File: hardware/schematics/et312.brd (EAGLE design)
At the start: 160 x 100 mm, 119 parts, among them IC1 LM324N, IC2 4066N, IC3 LM358, IC4 7809, IC5 LM358N, IC6 7809, J1 BATTERY_CONNDEANS, Q1 IRL520N-H, Q2 IRL520N-H, Q3 IRF9Z24, Q4 IRL520N-H, Q5 IRL520N-H, Q6 IRF9Z24, Q7 2N3906, T1 2N3904, U1 MEGA16-P, U9 7805, X1 HD44780LCD-1602, X2 STEREOJACK, X3 STEREOJACK, X4 STEREOJACK, X5 STEREOJACK, X6 STEREOJACK

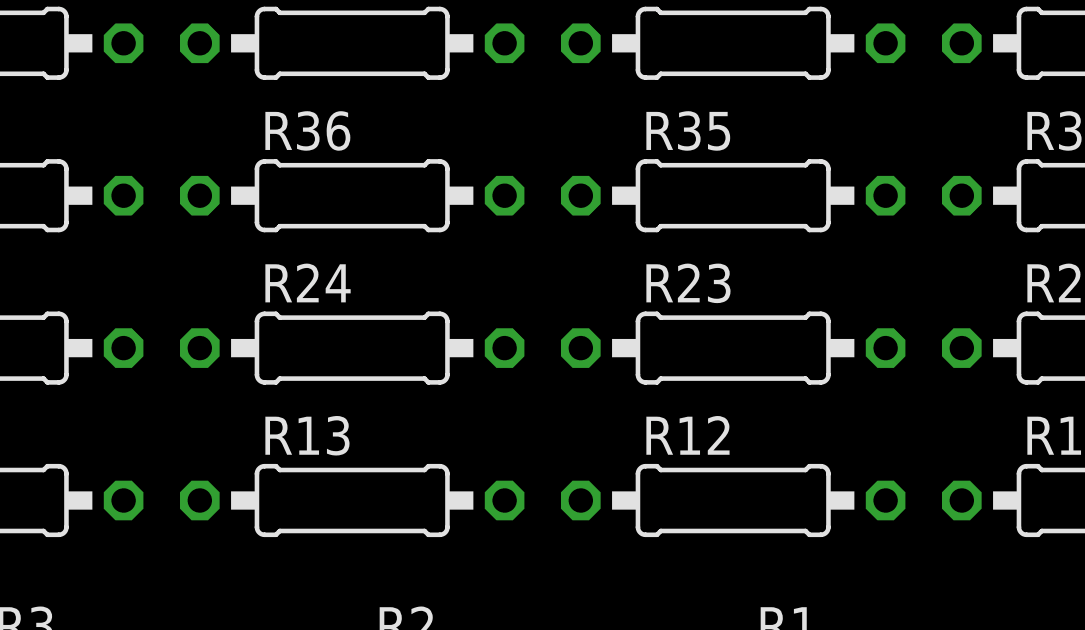
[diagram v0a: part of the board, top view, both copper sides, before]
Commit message: Arduino Sheild Eagle
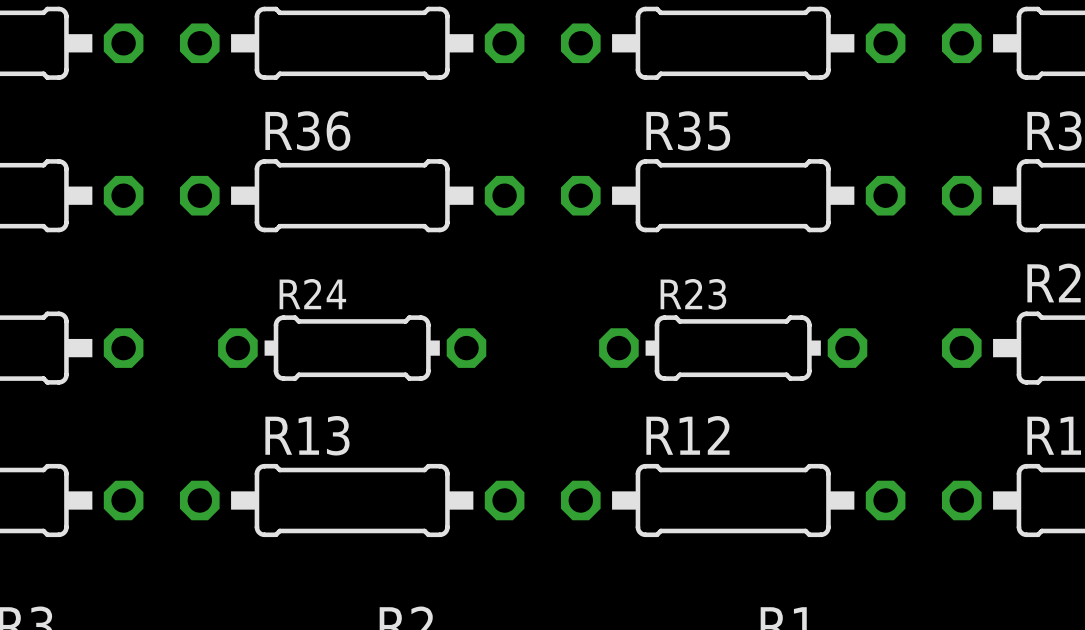
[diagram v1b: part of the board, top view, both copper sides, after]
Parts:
- R23, R24: device rcl:0207/10 -> rcl:0204/7
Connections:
- net +12V: no longer C7.+, L1.2
- net N$31: now also C7.+, L1.2; no longer L1.1
- net V+: now also L1.1
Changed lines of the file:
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@@
 <?xml version="1.0" encoding="utf-8"?>
 <!DOCTYPE eagle SYSTEM "eagle.dtd">
-<eagle version="7.3.0">
+<eagle version="7.1.0">
 <drawing>
 <settings>
@@
 <attribute name="SPICEPREFIX" value="R" x="-44.45" y="147.32" size="1.778" layer="27" display="off"/>
 </element>
-<element name="R23" library="rcl" package="0207/10" value="" x="-57.15" y="147.32"/>
-<element name="R24" library="rcl" package="0207/10" value="" x="-69.85" y="147.32"/>
+<element name="R23" library="rcl" package="0204/7" value="" x="-57.15" y="147.32"/>
+<element name="R24" library="rcl" package="0204/7" value="" x="-69.85" y="147.32"/>
 <element name="R25" library="pot" package="LI10" value="" x="-19.05" y="110.49"/>
 <element name="R26" library="rcl" package="0207/10" value="390R" x="-82.55" y="147.32"/>
@@
 <contactref element="IC1" pad="4"/>
 <contactref element="IC5" pad="8"/>
+<contactref element="RP6" pad="2"/>
 <contactref element="JP1" pad="PWR"/>
+<contactref element="U$1" pad="4"/>
 <contactref element="C5" pad="+"/>
-<contactref element="U$1" pad="4"/>
-<contactref element="RP6" pad="2"/>
-<wire x1="-71.12" y1="105.41" x2="-22.86" y2="125.73" width="0" layer="19" extent="1-1"/>
+<contactref element="L1" pad="1"/>
+<wire x1="-45.72" y1="135.89" x2="-22.86" y2="125.73" width="0" layer="19" extent="1-1"/>
+<wire x1="-64.77" y1="162.56" x2="-45.72" y2="135.89" width="0" layer="19" extent="1-1"/>
+<wire x1="-71.12" y1="105.41" x2="-45.72" y2="135.89" width="0" layer="19" extent="1-1"/>
 <wire x1="-101.6" y1="130.81" x2="-71.12" y2="105.41" width="0" layer="19" extent="1-1"/>
-<wire x1="-64.77" y1="162.56" x2="-101.6" y2="130.81" width="0" layer="19" extent="1-1"/>
 <wire x1="-99.02" y1="53.17" x2="-71.12" y2="105.41" width="0" layer="19" extent="1-1"/>
 <wire x1="-110.0582" y1="40.64" x2="-99.02" y2="53.17" width="0" layer="19" extent="1-1"/>
@@
 <contactref element="C4" pad="2"/>
 <contactref element="IC6" pad="2"/>
-<contactref element="JP1" pad="GND@1"/>
-<contactref element="JP1" pad="GND@2"/>
-<contactref element="C5" pad="-"/>
-<contactref element="U$1" pad="3"/>
-<contactref element="U$1" pad="2"/>
 <contactref element="R24" pad="1"/>
 <contactref element="C6" pad="-"/>
 <contactref element="C8" pad="2"/>
-<contactref element="J1" pad="-"/>
 <contactref element="C7" pad="-"/>
 <contactref element="U1" pad="11"/>
@@
 <contactref element="U$2" pad="1"/>
 <contactref element="R52" pad="1"/>
+<contactref element="JP1" pad="GND@2"/>
+<contactref element="JP1" pad="GND@1"/>
+<contactref element="U$1" pad="2"/>
+<contactref element="U$1" pad="3"/>
+<contactref element="C5" pad="-"/>
+<contactref element="J1" pad="-"/>
 <wire x1="-13.97" y1="152.4" x2="-13.97" y2="157.48" width="0" layer="19" extent="1-1"/>
 <wire x1="-24.13" y1="147.32" x2="-13.97" y2="152.4" width="0" layer="19" extent="1-1"/>
@@
 <wire x1="-62.23" y1="142.24" x2="-58.42" y2="135.89" width="0" layer="19" extent="1-1"/>
 <wire x1="-64.77" y1="152.4" x2="-62.23" y2="142.24" width="0" layer="19" extent="1-1"/>
-<wire x1="-74.93" y1="157.48" x2="-64.77" y2="152.4" width="0" layer="19" extent="1-1"/>
+<wire x1="-73.66" y1="147.32" x2="-64.77" y2="152.4" width="0" layer="19" extent="1-1"/>
+<wire x1="-74.93" y1="157.48" x2="-73.66" y2="147.32" width="0" layer="19" extent="1-1"/>
 <wire x1="-82.55" y1="162.56" x2="-74.93" y2="157.48" width="0" layer="19" extent="1-1"/>
-<wire x1="-74.93" y1="147.32" x2="-74.93" y2="157.48" width="0" layer="19" extent="1-1"/>
-<wire x1="-87.63" y1="147.32" x2="-74.93" y2="147.32" width="0" layer="19" extent="1-1"/>
+<wire x1="-87.63" y1="147.32" x2="-73.66" y2="147.32" width="0" layer="19" extent="1-1"/>
 <wire x1="-100.33" y1="152.4" x2="-87.63" y2="147.32" width="0" layer="19" extent="1-1"/>
 <wire x1="-113.03" y1="157.48" x2="-100.33" y2="152.4" width="0" layer="19" extent="1-1"/>
@@
 <contactref element="R24" pad="2"/>
 <contactref element="U$1" pad="1"/>
-<wire x1="-64.77" y1="147.32" x2="-62.23" y2="147.32" width="0" layer="19" extent="1-1"/>
-<wire x1="-115.1636" y1="40.64" x2="-64.77" y2="147.32" width="0" layer="19" extent="1-1"/>
+<wire x1="-66.04" y1="147.32" x2="-60.96" y2="147.32" width="0" layer="19" extent="1-1"/>
+<wire x1="-115.1636" y1="40.64" x2="-66.04" y2="147.32" width="0" layer="19" extent="1-1"/>
 </signal>
 <signal name="N$45">
@@
 <contactref element="C6" pad="+"/>
 <contactref element="D1" pad="A"/>
-<wire x1="-39.37" y1="130.81" x2="-52.07" y2="147.32" width="0" layer="19" extent="1-1"/>
-<wire x1="-112.268" y1="107.95" x2="-52.07" y2="147.32" width="0" layer="19" extent="1-1"/>
+<wire x1="-39.37" y1="130.81" x2="-53.34" y2="147.32" width="0" layer="19" extent="1-1"/>
+<wire x1="-112.268" y1="107.95" x2="-53.34" y2="147.32" width="0" layer="19" extent="1-1"/>
 <wire x1="-108.3564" y1="40.64" x2="-112.268" y2="107.95" width="0" layer="19" extent="1-1"/>
 </signal>
-<signal name="N$31">
-<contactref element="L1" pad="1"/>
-<contactref element="J1" pad="+"/>
-<wire x1="-29.21" y1="114.3" x2="-45.72" y2="135.89" width="0" layer="19" extent="1-1"/>
-</signal>
 <signal name="+12V">
-<contactref element="C7" pad="+"/>
 <contactref element="D1" pad="C"/>
-<contactref element="L1" pad="2"/>
 <contactref element="C8" pad="1"/>
 <contactref element="IC4" pad="1"/>
@@
 <contactref element="R40" pad="2"/>
 <wire x1="-33.02" y1="135.89" x2="-13.97" y2="162.56" width="0" layer="19" extent="1-1"/>
-<wire x1="-35.56" y1="135.89" x2="-33.02" y2="135.89" width="0" layer="19" extent="1-1"/>
-<wire x1="-49.53" y1="130.81" x2="-35.56" y2="135.89" width="0" layer="19" extent="1-1"/>
+<wire x1="-49.53" y1="130.81" x2="-33.02" y2="135.89" width="0" layer="19" extent="1-1"/>
 <wire x1="-73.66" y1="120.65" x2="-49.53" y2="130.81" width="0" layer="19" extent="1-1"/>
-<wire x1="-124.968" y1="107.95" x2="-73.66" y2="120.65" width="0" layer="19" extent="1-1"/>
 <wire x1="-40.64" y1="64.77" x2="-73.66" y2="120.65" width="0" layer="19" extent="1-1"/>
 <wire x1="-24.13" y1="64.77" x2="-40.64" y2="64.77" width="0" layer="19" extent="1-1"/>
-<wire x1="-130.81" y1="40.64" x2="-124.968" y2="107.95" width="0" layer="19" extent="1-1"/>
+<wire x1="-130.81" y1="40.64" x2="-40.64" y2="64.77" width="0" layer="19" extent="1-1"/>
 </signal>
 <signal name="+9V1">
@@
 <wire x1="-107.79" y1="92.61" x2="-138.43" y2="97.536" width="0" layer="19" extent="1-1"/>
 </signal>
+<signal name="N$31">
+<contactref element="J1" pad="+"/>
+<contactref element="C7" pad="+"/>
+<contactref element="L1" pad="2"/>
+<wire x1="-29.21" y1="114.3" x2="-35.56" y2="135.89" width="0" layer="19" extent="1-1"/>
+<wire x1="-124.968" y1="107.95" x2="-35.56" y2="135.89" width="0" layer="19" extent="1-1"/>
+</signal>
 </signals>

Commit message: Pin Swap
et312.sch page 6 vs 03_output_stage_1.gif, bottom opamp (pins 5 & 6)
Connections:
- net N$28: now also IC3.5; no longer IC3.6
- net N$41: now also IC3.6; no longer IC3.5
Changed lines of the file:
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@@
 <?xml version="1.0" encoding="utf-8"?>
 <!DOCTYPE eagle SYSTEM "eagle.dtd">
-<eagle version="7.1.0">
+<eagle version="7.3.0">
 <drawing>
 <settings>
@@
 </signal>
 <signal name="N$28">
+<contactref element="R18" pad="1"/>
 <contactref element="R17" pad="2"/>
-<contactref element="R18" pad="1"/>
-<contactref element="IC3" pad="6"/>
+<contactref element="IC3" pad="5"/>
 <contactref element="R22" pad="2"/>
 <wire x1="-115.57" y1="142.24" x2="-39.37" y2="147.32" width="0" layer="19" extent="1-1"/>
 <wire x1="-138.43" y1="142.24" x2="-115.57" y2="142.24" width="0" layer="19" extent="1-1"/>
-<wire x1="-133.35" y1="111.76" x2="-138.43" y2="142.24" width="0" layer="19" extent="1-1"/>
+<wire x1="-130.81" y1="111.76" x2="-138.43" y2="142.24" width="0" layer="19" extent="1-1"/>
 </signal>
 <signal name="N$33">
@@
 <contactref element="R16" pad="1"/>
 <contactref element="R19" pad="1"/>
-<contactref element="IC3" pad="5"/>
 <contactref element="R20" pad="2"/>
+<contactref element="IC3" pad="6"/>
 <wire x1="-113.03" y1="142.24" x2="-13.97" y2="147.32" width="0" layer="19" extent="1-1"/>
-<wire x1="-130.81" y1="111.76" x2="-113.03" y2="142.24" width="0" layer="19" extent="1-1"/>
-<wire x1="-151.13" y1="142.24" x2="-130.81" y2="111.76" width="0" layer="19" extent="1-1"/>
+<wire x1="-133.35" y1="111.76" x2="-113.03" y2="142.24" width="0" layer="19" extent="1-1"/>
+<wire x1="-151.13" y1="142.24" x2="-133.35" y2="111.76" width="0" layer="19" extent="1-1"/>
 </signal>
 <signal name="N$42">
